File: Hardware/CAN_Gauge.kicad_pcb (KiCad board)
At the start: 2 copper layers, 50 x 50 mm, 77 parts, among them J1 Conn_02x03_Odd_Even, J2 Conn_01x08, SW1 SW_Push, U1 STM32F042K6Tx, U2 SN65HVD230, U3 2594, U4 UG-2864HSWEG01

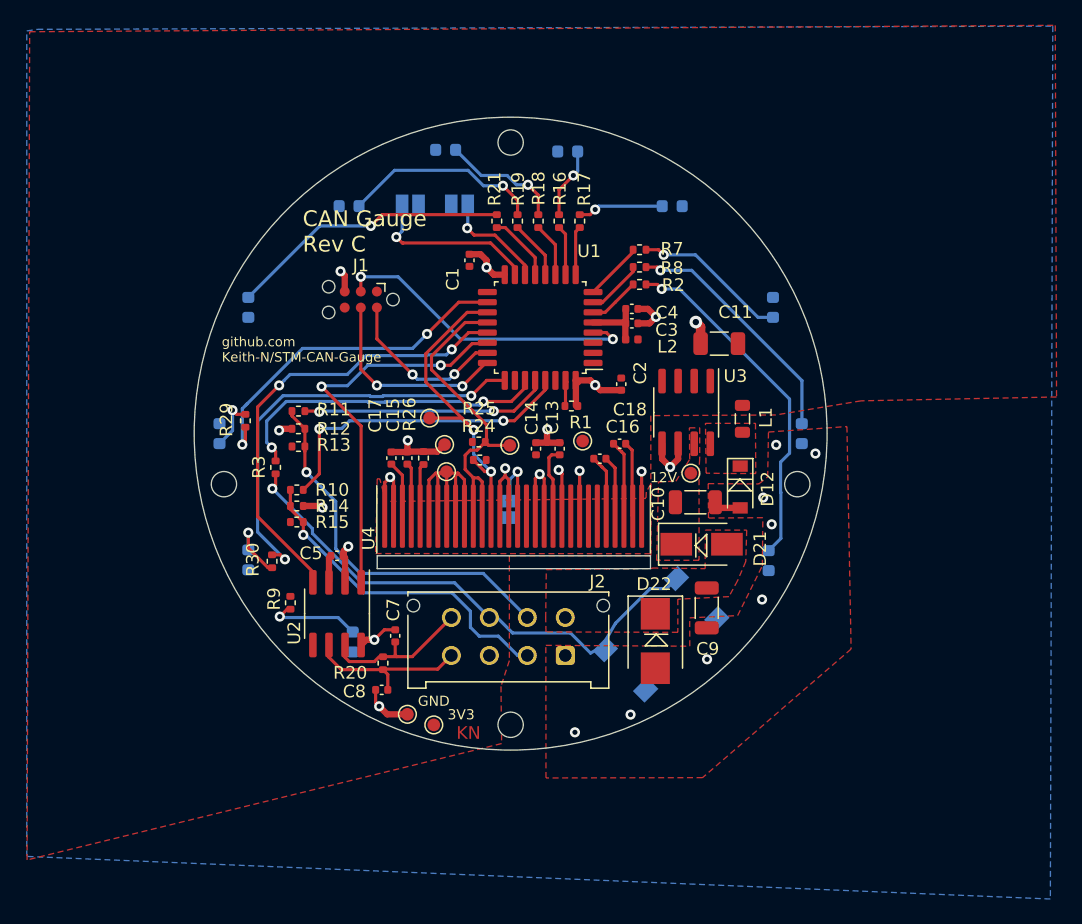
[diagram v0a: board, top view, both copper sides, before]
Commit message: Update for F103
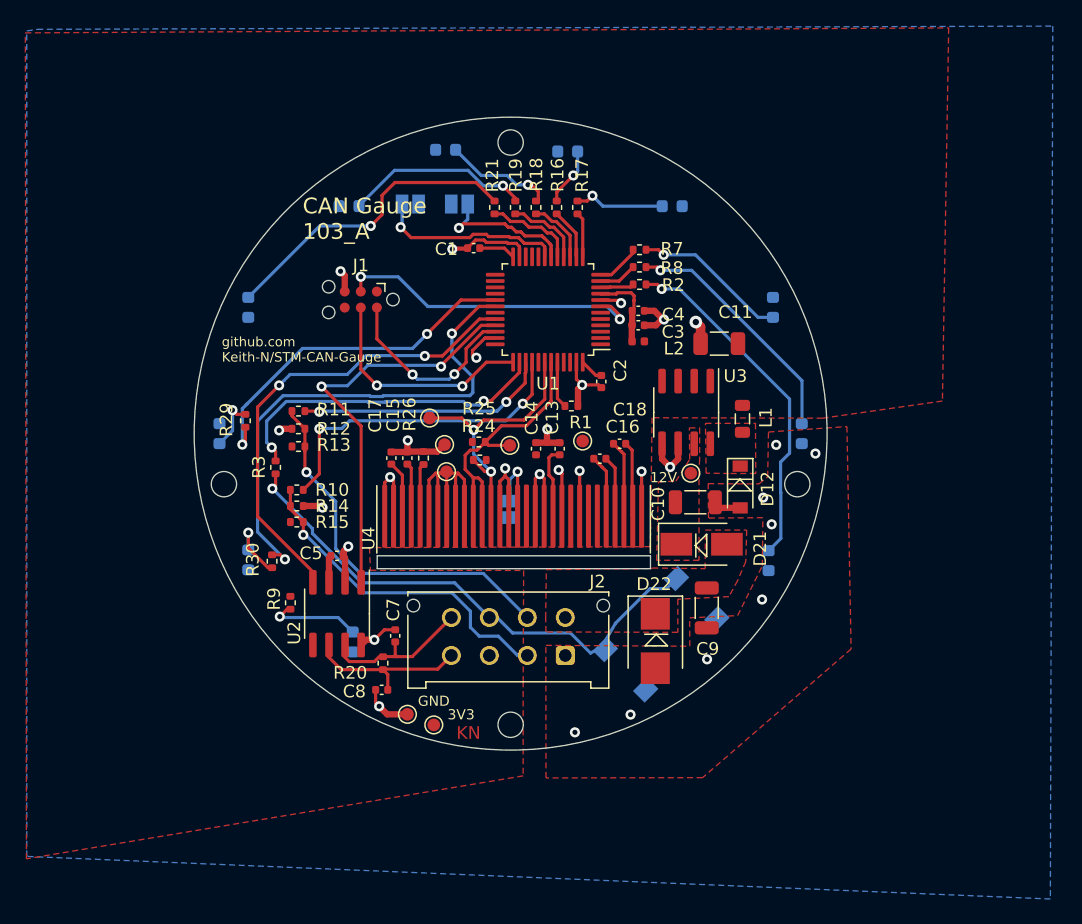
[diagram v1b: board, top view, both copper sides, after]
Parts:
- U1: value STM32F042K6Tx -> STM32F103C8Tx; footprint Package_QFP:LQFP-32_7x7mm_P0.8mm -> Package_QFP:LQFP-48_7x7mm_P0.5mm
- moved C2 1.59 mm to (140.5, 90.5)
- moved U1 1.55 mm to (136.3, 84.8)
- moved R18 1.09 mm to (135.3, 76.7)
- moved R21 1.09 mm to (132.0, 76.7)
- moved R16 1.09 mm to (136.9, 76.7)
- moved R17 1.09 mm to (138.6, 76.7)
- moved R19 1.09 mm to (133.7, 76.7)
- moved C1 1.02 mm to (130.4, 79.9), turned to 180 degrees
- moved C3 0.53 mm to (143.4, 86.0)
- moved C4 0.53 mm to (143.4, 84.9)
- moved L2 0.53 mm to (143.4, 87.3)
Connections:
- net Net-(U1-Pad3) renamed OSC_IN
- U1 pad 1: +3V3 -> Net-(U1-Pad1)
- U1 pad 10: LED5 -> LED1
- U1 pad 11: LED6 -> LED2
- U1 pad 12: LED7 -> LED3
- U1 pad 13: LED8 -> LED4
- U1 pad 14: /STM/CONFIG_1 -> LED5
- U1 pad 15: /STM/CONFIG_2 -> LED6
- U1 pad 16: GND -> LED7
- U1 pad 17: +3V3 -> LED8
- U1 pad 18: LED9 -> /STM/CONFIG_1
- U1 pad 19: I2C1_SCL -> /STM/CONFIG_2
- U1 pad 20: I2C1_SDA -> Net-(U1-Pad20)
- U1 pad 21: CAN_RX -> Net-(U1-Pad21)
- U1 pad 22: CAN_TX -> Net-(U1-Pad22)
- U1 pad 23: SWDIO -> GND
- U1 pad 24: SWCLK -> +3V3
- U1 pad 25: LED10 -> Net-(U1-Pad25)
- U1 pad 27: USER_INPUT -> Net-(U1-Pad27)
- U1 pad 28: SPARE_1_IN -> Net-(U1-Pad28)
- U1 pad 29: SPARE_2_IN -> LED9
- U1 pad 30: Net-(U1-Pad30) -> LED10
- U1 pad 31: BOOT0 -> Net-(U1-Pad31)
- U1 pad 32: GND -> CAN_RX
- U1 pad 4: NRST -> OSC_OUT
- U1 pad 5: VDDA -> Net-(U1-Pad5)
- U1 pad 6: LED1 -> Net-(U1-Pad6)
- U1 pad 7: LED2 -> NRST
- U1 pad 8: LED3 -> GND
- U1 pad 9: LED4 -> VDDA
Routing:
- net GND: track 75.6 -> 84.2 mm, vias 27 -> 29
- net LED10: track 33.9 -> 40.6 mm
- net +3V3: track 14.4 -> 19.2 mm
- net I2C1_SDA: track 26.8 -> 22.5 mm
- net I2C1_SCL: track 29.2 -> 25.0 mm
- net /STM/CONFIG_1: track 8.45 -> 11.3 mm
- net Net-(D8-Pad2): track 22.3 -> 24.7 mm
- net SWCLK: track 16.3 -> 18.3 mm
- net SWDIO: track 13.4 -> 15.3 mm
- net LED8: track 5.37 -> 7.20 mm
- net BOOT0: track 2.23 -> 3.77 mm
- net VDDA: track 5.04 -> 6.57 mm
- net LED7: track 4.63 -> 6.14 mm
- net LED2: track 4.52 -> 3.02 mm
- net LED1: track 4.08 -> 2.66 mm
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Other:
- board text added: "CAN Gauge 103_A"
- board text removed: "CAN Gauge Rev C"
